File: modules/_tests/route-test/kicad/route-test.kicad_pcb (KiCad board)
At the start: 2 copper layers, 40 x 32 mm, 8 parts, among them J1 LEFT, J2 RIGHT

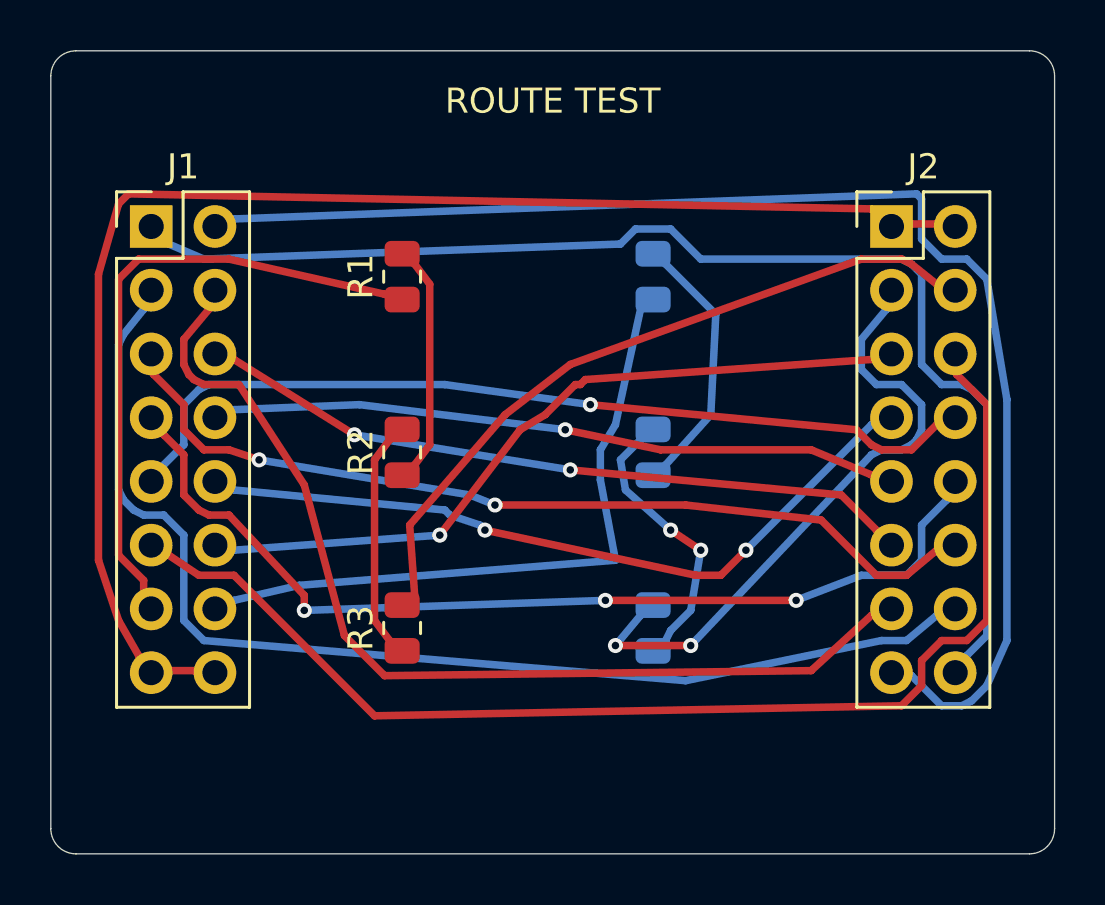
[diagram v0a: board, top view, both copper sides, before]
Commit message: M1-M3: reject invalid designs, forbid vias in pads, fail closed on export
Three of the roadmap's review findings become code and tests. Every design
is now validated before emission, the router's result is checked on the
final geometry rather than trusted, and nothing can be exported that a
clean check did not produce.

Validation (toolkit/src/Validate.hs, wired into pcbgen before emission):
unique references and net names, every (ref, pin) must exist on the library
symbol, every symbol pin must be on exactly one net or listed in the new
partNoConnect, assembly class and LCSC field must agree, dimensions and
routing settings must be positive. On any diagnostic pcbgen prints them and
exits 1 without writing a file. The four wiring faults ERC used to accept
(U1.8 removed, mistyped as U1.88, on both rails, D2.1 dropped) are rejected
with diagnostics that name the pin.

Routing (toolkit/src/Route/Check.hs, Router.hs): a via may no longer be
placed in or against any pad, its own net included, which is what put 0.3 mm
drills in four SMD solder lands. Pre-routed copper is treated as one terminal
per island, so a hand-drawn trace can no longer make a net look finished
while a pad hangs unconnected, and it now blocks by its own width. Per-net
connectivity and via/pad clearance are recomputed on the emitted geometry;
any failure, contested cell or disconnect aborts generation.

Pours: Zone gains an explicit PadConnect. The attenuverter routes GND as
copper, so its pours no longer bond to pads at all, which also removes the
starved-thermal violation the stricter routing exposed. The mult's sleeves
are held by its pours alone and keep thermal relief; validation rejects an
unbonded pour on a net nothing routes.

Scripts: check.sh writes build/check.ok (tool versions, git provenance,
sha256 of every source and of the zone-filled board) only when ERC and DRC
are both clean, and removes stale copies first. fab.sh refuses unless every
hash still matches, builds into a temporary dire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
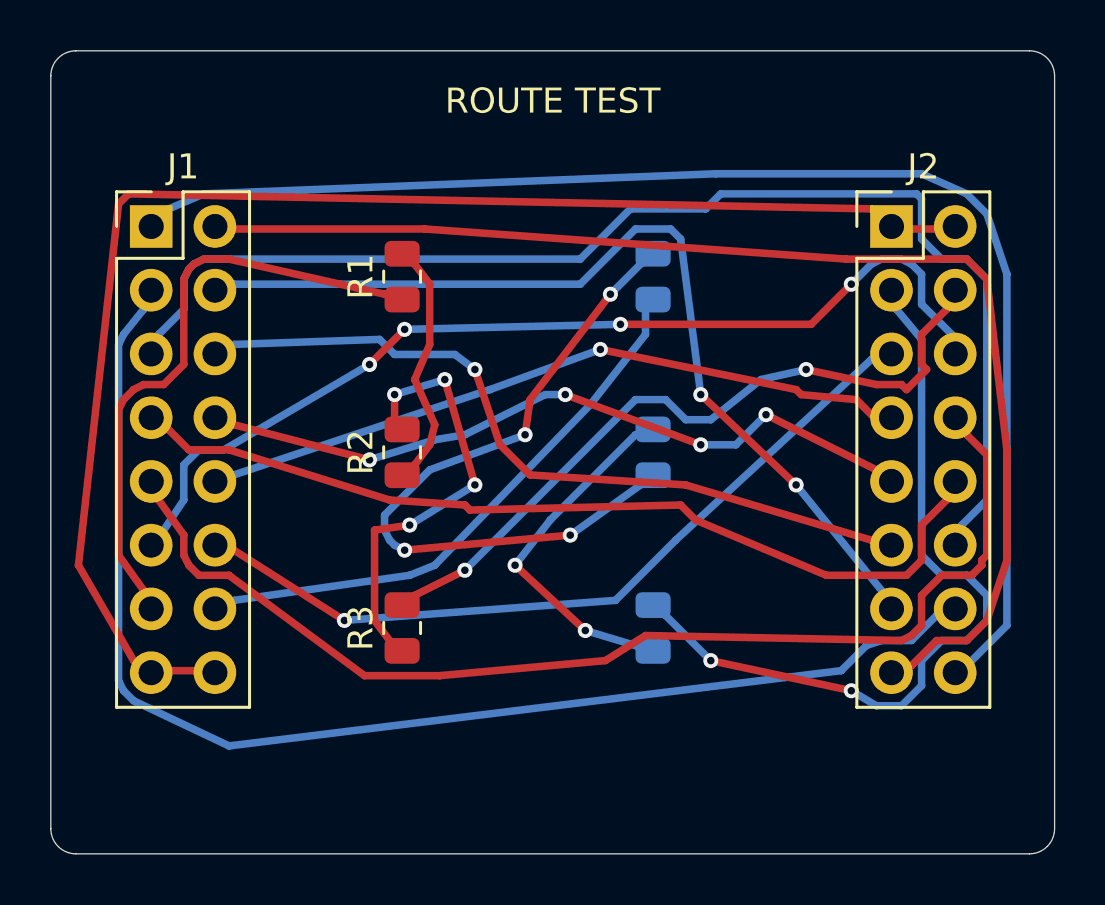
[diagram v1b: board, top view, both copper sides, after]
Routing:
- net /RF: track 10.8 -> 28.1 mm, vias 0 -> 4
- net /X5: track 36.2 -> 50.3 mm, vias 2 -> 0
- net /X9: track 35.5 -> 45.5 mm, vias 1 -> 0
- net /X11: track 49.1 -> 39.7 mm, vias 0 -> 4
- net /RC: track 9.70 -> 17.7 mm, vias 0 -> 4
- net /RH: track 25.6 -> 31.7 mm
- net /X2: track 54.2 -> 49.5 mm
- net /X3: track 46.8 -> 51.2 mm
- net /RE: track 27.1 -> 22.9 mm
- net /X1: track 50.1 -> 53.6 mm
- net /X7: track 39.3 -> 36.1 mm, vias 3 -> 0
- net /RG: track 11.5 -> 14.5 mm
- net /X4: track 40.3 -> 37.4 mm, vias 0 -> 2
- net /X8: track 27.4 -> 29.2 mm, vias 1 -> 4
- net /X12: track 29.9 -> 31.7 mm
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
